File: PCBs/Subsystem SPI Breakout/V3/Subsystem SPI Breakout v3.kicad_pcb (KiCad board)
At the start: 2 copper layers, 80 x 50.5 mm, 19 parts

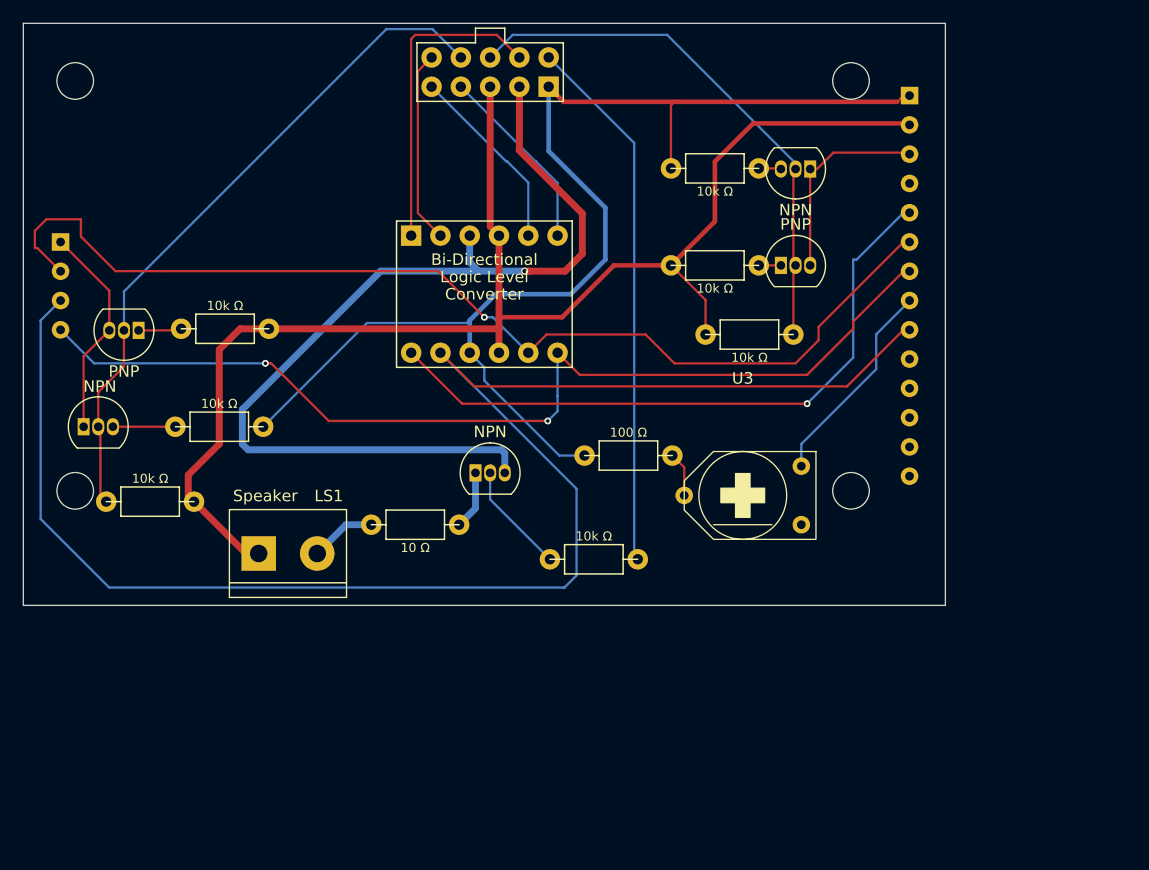
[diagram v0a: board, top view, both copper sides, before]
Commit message: Finished SPI Breakout Board V3
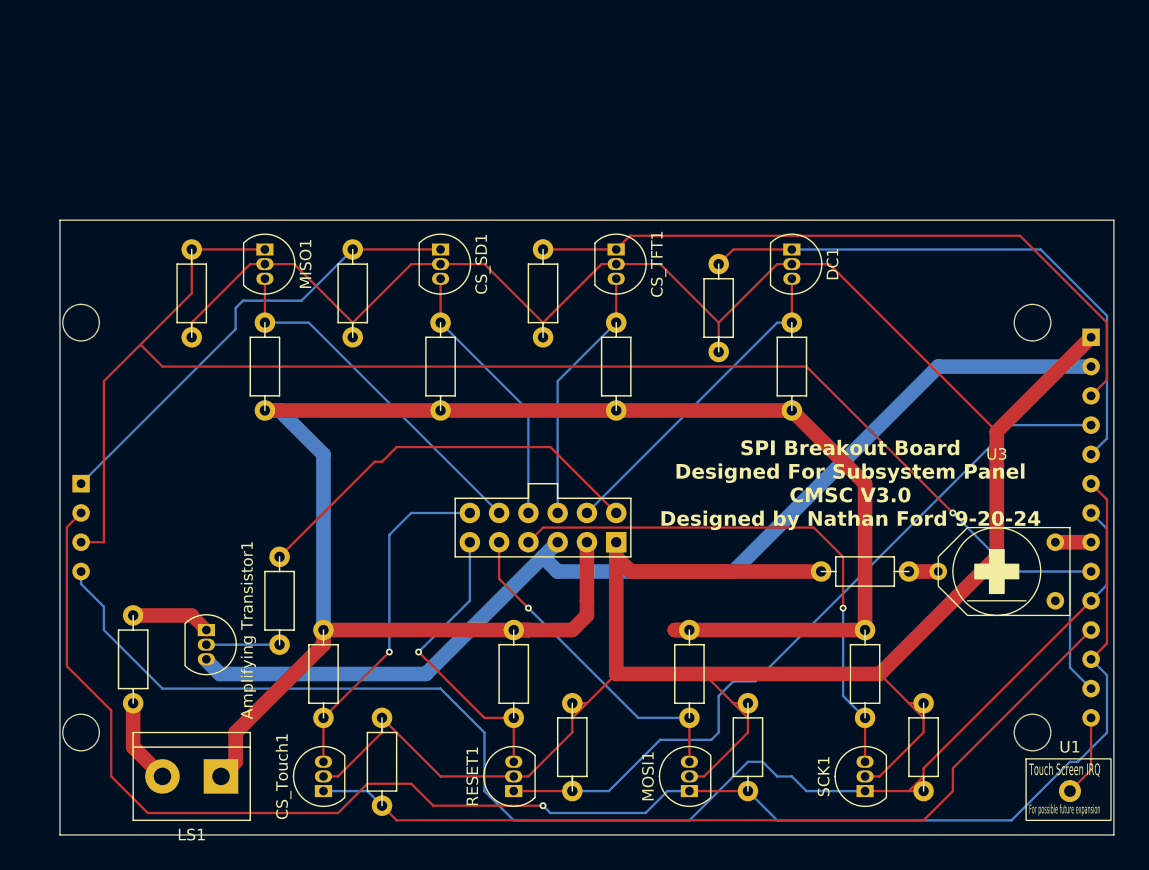
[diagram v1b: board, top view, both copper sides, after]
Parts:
- removed 1: ~, Subsystem Main:SPI_HEADER_RIBBON_CONNECTOR
- removed LogicConverter1: ~, Subsystem Main:BI_DIRECTIONAL_LOGIC_LEVEL_CONVERTER
- removed NPN (x3): NPN transistor, Package_TO_SOT_THT:TO-92_Inline
- removed PNP (x2): PNP Transistor, Package_TO_SOT_THT:TO-92_Inline
- added Amplifying Transistor1: NPN transistor, Package_TO_SOT_THT:TO-92_Inline, F.Cu at (119.4, 104.1)
- added C1: ~, Subsystem Main Extra Symbols:SPI_HEADER_RIBBON_CONNECTOR_V2, F.Cu at (148.6, 95.2)
- added CS_SD1: BS170, Package_TO_SOT_THT:TO-92_Inline, F.Cu at (139.7, 71.1)
- added CS_TFT1: BS170, Package_TO_SOT_THT:TO-92_Inline, F.Cu at (154.9, 71.1)
- added CS_Touch1: BS170, Package_TO_SOT_THT:TO-92_Inline, F.Cu at (129.5, 118.1)
- added DC1: BS170, Package_TO_SOT_THT:TO-92_Inline, F.Cu at (170.2, 71.1)
- added MISO1: BS170, Package_TO_SOT_THT:TO-92_Inline, F.Cu at (124.5, 71.1)
- added MOSI1: BS170, Package_TO_SOT_THT:TO-92_Inline, F.Cu at (161.3, 118.1)
- added R10: 10k Ω, Subsystem Main:THROUGH_HOLE_RESISTOR, F.Cu at (148.6, 74.9)
- added R11: 10k Ω, Subsystem Main:THROUGH_HOLE_RESISTOR, F.Cu at (154.9, 81.3)
- added R12: 10k Ω, Subsystem Main:THROUGH_HOLE_RESISTOR, F.Cu at (163.8, 76.2)
- added R13: 10k Ω, Subsystem Main:THROUGH_HOLE_RESISTOR, F.Cu at (170.2, 81.3)
- added R14: 10k Ω, Subsystem Main:THROUGH_HOLE_RESISTOR, F.Cu at (132.1, 74.9)
- added R15: 10k Ω, Subsystem Main:THROUGH_HOLE_RESISTOR, F.Cu at (139.7, 81.3)
- added R16: 10k Ω, Subsystem Main:THROUGH_HOLE_RESISTOR, F.Cu at (134.6, 115.6)
- added R17: 10k Ω, Subsystem Main:THROUGH_HOLE_RESISTOR, F.Cu at (129.5, 108.0)
- added R18: 10k Ω, Subsystem Main:THROUGH_HOLE_RESISTOR, F.Cu at (151.1, 114.3)
- added R19: 10k Ω, Subsystem Main:THROUGH_HOLE_RESISTOR, F.Cu at (146.1, 108.0)
- added RESET1: BS170, Package_TO_SOT_THT:TO-92_Inline, F.Cu at (146.1, 118.1)
- added SCK1: BS170, Package_TO_SOT_THT:TO-92_Inline, F.Cu at (176.5, 118.1)
- added U1: ~, Subsystem Main Extra Symbols:T_IRQ, F.Cu at (194.3, 118.1)
- U2: footprint Subsystem Main:2.4'_TFT_SPI_ILI9341_WITH_SD_CARD -> Subsystem Main:2.8__TFT_SPI_ILI9341_WITH_SD_CARD
- moved U2 60.2 mm to (198.7, 95.2)
- moved R2 60.0 mm to (176.5, 108.0), turned to -90 degrees
- moved R3 58.1 mm to (166.4, 114.3), turned to -90 degrees
- moved R1 53.4 mm to (181.6, 114.3), turned to -90 degrees
- moved R6 42.1 mm to (124.5, 81.3), turned to 90 degrees
- moved R4 35.5 mm to (161.3, 108.0), turned to -90 degrees
- moved R8 27.5 mm to (125.7, 101.6), turned to 90 degrees
- moved R7 27.1 mm to (113.0, 106.7), turned to -90 degrees
- moved U3 23.0 mm to (188.0, 99.1)
- moved R9 22.9 mm to (176.5, 99.1)
- moved LS1 19.6 mm to (120.7, 116.8), turned to 180 degrees
- moved R5 18.4 mm to (118.1, 74.9), turned to 90 degrees
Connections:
- LS1 pad 1: Net-(1-PadGND) -> /5V
- R1 pad P$1: Net-(Q2-C) -> /3V3
- R1 pad P$2: Net-(1-Pad3V3) -> /SCK_3V3
- R2 pad P$1: Net-(Q4-C) -> /5V
- R2 pad P$2: Net-(1-Pad3V3) -> /SCK_5V
- R3 pad P$1: Net-(Q3-E) -> /3V3
- R3 pad P$2: Net-(1-PadGND) -> /MOSI_3V3
- R4 pad P$1: Net-(Q1-E) -> /5V
- R4 pad P$2: Net-(1-PadGND) -> /MOSI_5V
- R5 pad P$1: Net-(Q3-B) -> /3V3
- R5 pad P$2: Net-(1-PadGND) -> /MISO_3V3
- R6 pad P$1: Net-(Q1-B) -> /5V
- R6 pad P$2: Net-(1-PadGND) -> /MISO_5V
- R9 pad P$1: Net-(1-Pad3V3) -> /3V3
- U2 pad CS: Net-(Q1-C) -> /CS_TFT_3V3
- U2 pad DC: Net-(LogicConverter1-PadLV1) -> /DC_3V3
- U2 pad GND: Net-(1-PadGND) -> /GND
- U2 pad RESET: unconnected-(U2-PadRESET) -> /RESET_3V3
- U2 pad SCK: Net-(LogicConverter1-PadLV4) -> /SCK_3V3
- U2 pad SDI(MOSI): Net-(LogicConverter1-PadLV3) -> /MOSI_3V3
- U2 pad SDO(MISO): Net-(LogicConverter1-PadLV2) -> /MISO_3V3
- U2 pad SD_CS: Net-(Q3-C) -> /CS_SD_3V3
- U2 pad SD_MISO: Net-(LogicConverter1-PadLV2) -> /MISO_3V3
- U2 pad SD_MOSI: Net-(LogicConverter1-PadLV3) -> /MOSI_3V3
- U2 pad SD_SCK: Net-(LogicConverter1-PadLV4) -> /SCK_3V3
- U2 pad T_CLK: unconnected-(U2-PadT_CLK) -> /SCK_3V3
- U2 pad T_CS: unconnected-(U2-PadT_CS) -> /CS_TOUCH_3V3
- U2 pad T_DIN: unconnected-(U2-PadT_DIN) -> /MOSI_3V3
- U2 pad T_DO: unconnected-(U2-PadT_DO) -> /MISO_3V3
- U2 pad T_IRQ: unconnected-(U2-PadT_IRQ) -> Net-(U1-T_IRQ)
- U2 pad Vcc: Net-(1-Pad3V3) -> /3V3
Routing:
- net /3V3: track 0.00 -> 255.4 mm
- net /5V: track 0.00 -> 154.5 mm
- net /MOSI_3V3: track 0.00 -> 143.1 mm, vias 0 -> 1
- net /MISO_3V3: track 0.00 -> 138.4 mm, vias 0 -> 1
- net Net-(LogicConverter1-PadLV2): track 137.0 -> 0.00 mm
- net /SCK_3V3: track 0.00 -> 124.0 mm
- net Net-(1-PadGND): track 122.9 -> 0.00 mm
- net Net-(1-Pad3V3): track 108.8 -> 0.00 mm
- net Net-(LogicConverter1-PadLV3): track 93.0 -> 0.00 mm, vias 1 -> 0
- net /GND: track 0.00 -> 91.1 mm
- net Net-(LogicConverter1-PadLV4): track 86.9 -> 0.00 mm, vias 2 -> 0
- net Net-(Q5-C): track 83.9 -> 0.00 mm, vias 1 -> 0
- net /CS_TOUCH_3V3: track 0.00 -> 75.7 mm
- net /RESET_3V3: track 0.00 -> 66.4 mm
- net /CS_TFT_3V3: track 0.00 -> 59.5 mm
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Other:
- board size 80 x 50.5 mm -> 91.4 x 53.3 mm
- board text added: "SPI Breakout Board Designed For Subsystem Panel CMSC V3.0 Designed by Nathan Ford 9-20-24"
